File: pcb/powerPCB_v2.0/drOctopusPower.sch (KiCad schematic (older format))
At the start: 74 parts, among them CON1 Servo, CON10 AVR_Prog, CON2 Servo, CON3 Heater, CON4 +12V, CON5 BEC, CON6 PIN-2x2_angled, CON7 FAN1, CON8 FAN2, CON9 UART, Q1 16MHz, SW1 RESET, T1 IRLR2905PBF, T2 IRLML6244TRPBF, T3 IRLML6244TRPBF, T4 IRLML6244TRPBF, U1 ATmega328-AU, U2 78M05CDT, U3 ESP-01, U4 AMS1117-3.3

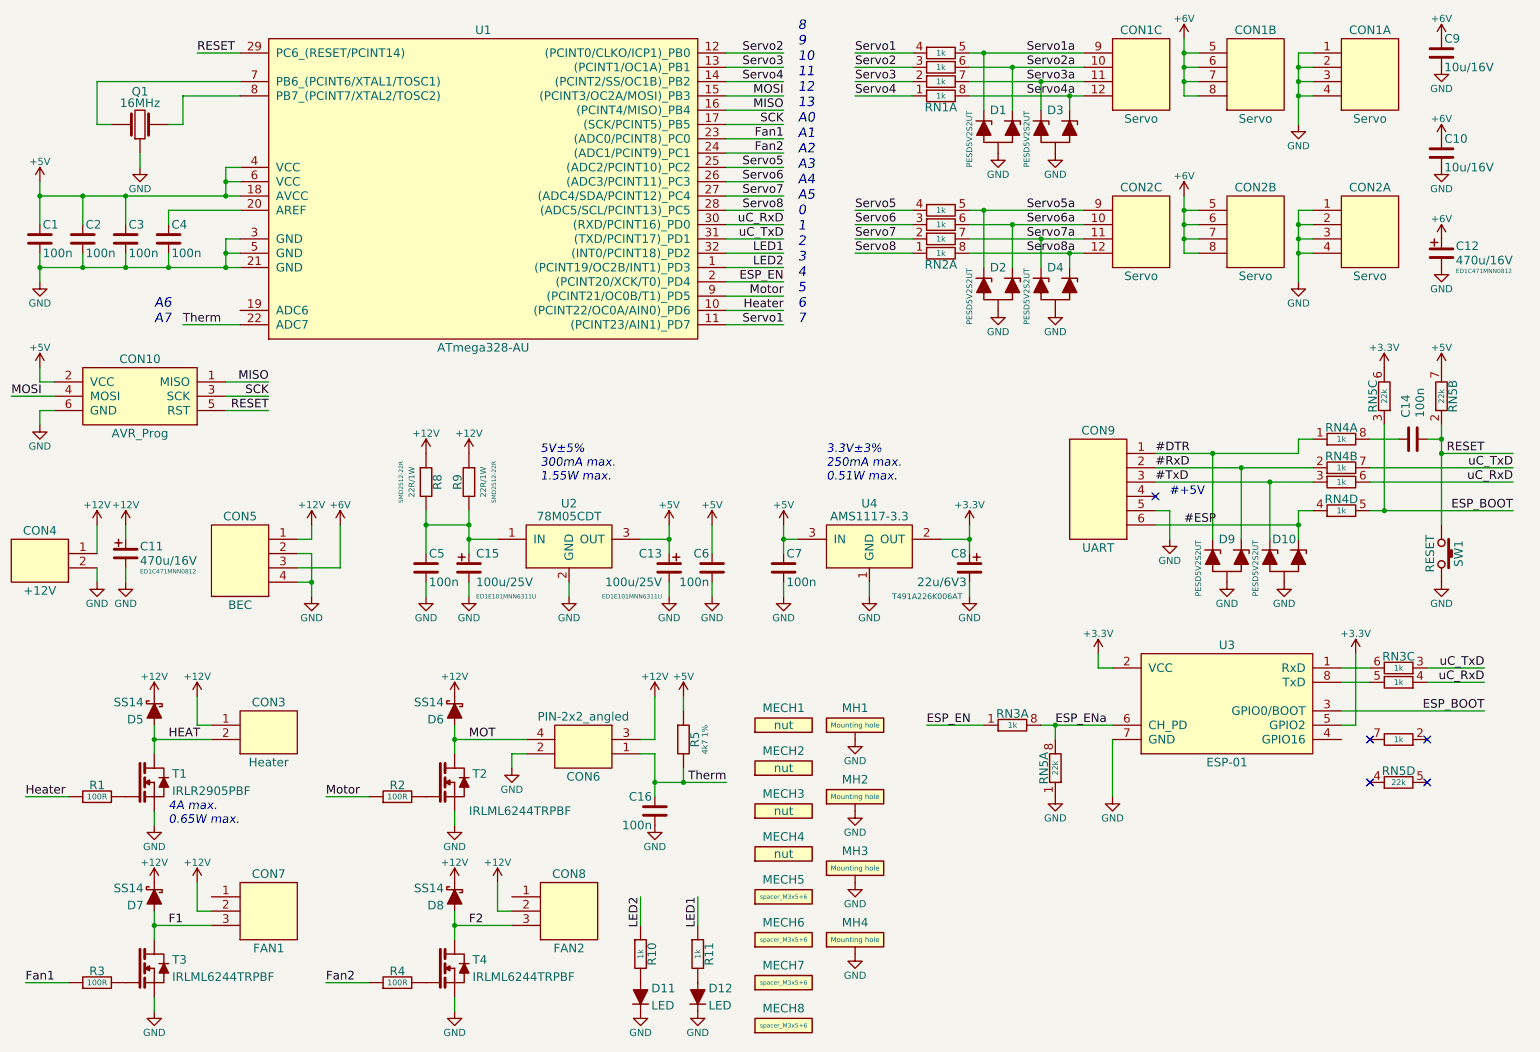
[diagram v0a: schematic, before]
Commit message: Working on Power PCB
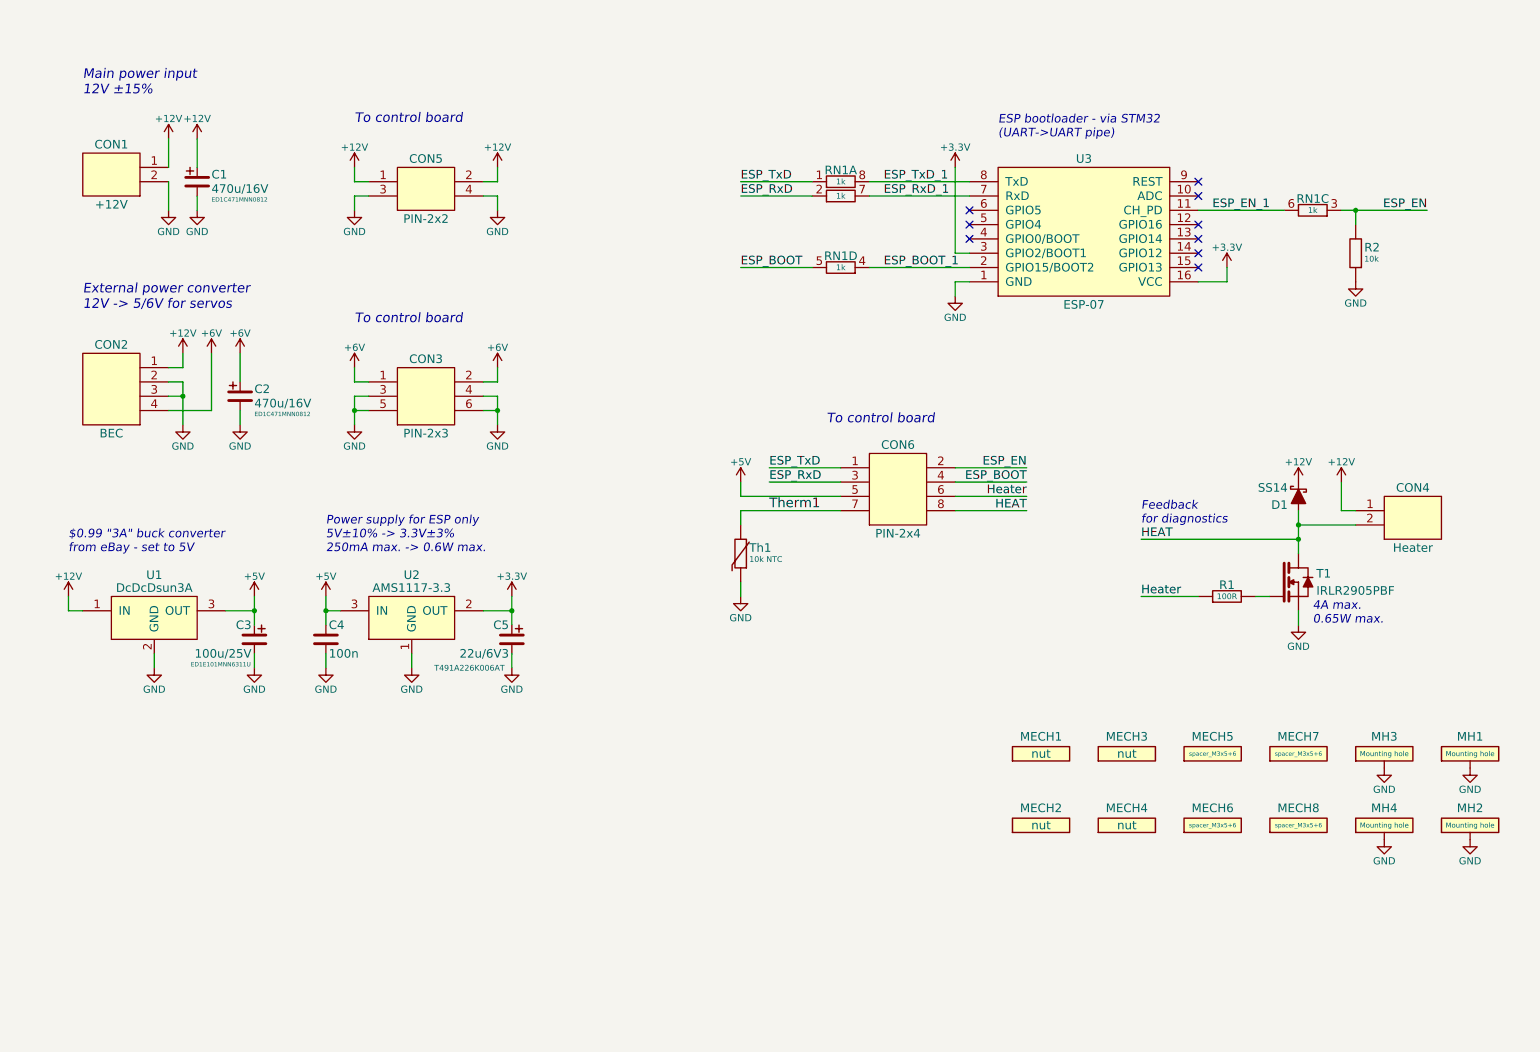
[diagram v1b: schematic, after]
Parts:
- removed C1, C14, C16, C2, C3, C4, C5, C6: 100n, 0603_N, symbol C
- removed C10, C9: 10u/16V, 0805_N, symbol C
- removed C12: 470u/16V, Cpol_8.0_12.0_M, symbol Cpol
- removed C13, C15: 100u/25V, Cpol_6.3_11.0_N, symbol Cpol
- removed CON1, CON2: Servo, PIN-3x4_angled_N, symbol PIN-3x4
- removed CON10: AVR_Prog, PIN-2x3_N, symbol AVR_Prog
- removed CON6: PIN-2x2_angled, PIN-2x2_angled_N, symbol PIN-2x2_angled
- removed CON7: FAN1, PIN-1x3_M, symbol PIN-1x3
- removed CON8: FAN2, PIN-1x3_M, symbol PIN-1x3
- removed CON9: UART, PIN-1x6_angled_N, symbol PIN-1x6_angled
- removed D1, D10, D2, D3, D4, D9: PESD5V2S2UT, SOT23-3_N, symbol PESD5V2S2UT
- removed D11, D12: LED, 0805_N, symbol diode
- removed D6, D7, D8: SS14, SMA_N, symbol SS14
- removed Q1: 16MHz, 3.7x3.1_N, symbol Ceramic_3.7x3.1_16MHz
- removed R10, R11: 1k, 0603_N, symbol R
- removed R2, R3, R4: 100R, 0603_N, symbol R
- removed R5: 4k7 1%, 0603_N, symbol R
- removed R8, R9: 22R/1W, 2512_N, symbol R
- removed RN1, RN2, RN4: 1k, 4x0603_N, symbol R_Network_4
- removed RN5: 22k, 4x0603_N, symbol R_Network_4
- removed SW1: RESET, MicroswitchSmd-4.3_N, symbol MicroswitchSmt-4.3
- removed T2, T3, T4: IRLML6244TRPBF, SOT23-3_N, symbol IRLML6244TRPBF
- removed U1: ATmega328-AU, QFP-32-0.8_M, symbol ATmega328-AU
- removed U2: 78M05CDT, D-PAK_N, symbol 78M05CDT
- removed U3: ESP-01, ESP-01_N_socket, symbol ESP-01
- added C2: 470u/16V, niceRLC:Cpol_8.0_12.0_HR_N, symbol Cpol
- added C3: 100u/25V, niceRLC:Cpol_6.3_11.0_HR_N, symbol Cpol
- added CON3: PIN-2x3, PIN-2x3_N, symbol PIN-2x3
- added CON5: PIN-2x2, PIN-2x2_N, symbol PIN-2x2
- added CON6: PIN-2x4, nicePinheaders:PIN-2x4_N, symbol PIN-2x4
- added R2: 10k, 0603_N, symbol R_V
- added Th1: 10k NTC, 0603_N, symbol Thermistor_V
- added U1: DcDcDsun3A, niceModules:DcDcDsun3A_5.08N, symbol DcDcDsun3A
- added U3: ESP-07, ESP-07_N, symbol ESP-07
- C1: renamed from C11; footprint Cpol_8.0_12.0_M -> niceRLC:Cpol_8.0_12.0_HR_N
- renumbered C7 to C4, C8 to C5, CON4 to CON1, CON5 to CON2, CON3 to CON4, D5 to D1, RN3 to RN1, U4 to U2
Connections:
- net +12V: now also CON5.1, CON5.2, U1.1 (IN)
- net +3V3: now also U3.16 (VCC), U3.3 (GPIO2/BOOT1)
- net +5V: now also C3.1, CON6.5, U1.3 (OUT)
- net +6V: now also CON2.4, C2.1, CON3.1, CON3.2; no longer CON2.3
- net ESP_BOOT: now also RN1.5 (2), CON6.4
- net ESP_EN: now also RN1.3 (1), CON6.2, R2.2; no longer RN1.1
- net GND: now also CON2.3, C2.2, C3.2, CON3.3, CON3.4, CON3.5, CON3.6, CON5.3, CON5.4, R2.1, Th1.1, U1.2 (GND), U3.1 (GND); no longer CON2.4
- net HEAT: now also CON6.8
- net Heater: now also CON6.6
- removed net ESP_ENa: RN1.8 (2)
- removed net uC_RxD: RN1.4 (1)
- removed net uC_TxD: RN1.3 (1)
- new net ESP_BOOT_1: RN1.4 (1), U3.2 (GPIO15/BOOT2)
- new net ESP_EN_1: RN1.6 (2), U3.11 (CH_PD)
- new net ESP_RxD: CON6.3, RN1.2 (1)
- new net ESP_RxD_1: RN1.7 (2), U3.7 (RxD)
- new net ESP_TxD: CON6.1, RN1.1
- new net ESP_TxD_1: RN1.8 (2), U3.8 (TxD)
- new net Therm1: CON6.7, Th1.2
- no-connect marks 5 -> 9
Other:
- note added: "$0.99 "3A" buck converter\nfrom eBay - set to 5V"
- note added: "ESP bootloader - via STM32 \n(UART->UART pipe)"
- note added: "External power converter\n12V -> 5/6V for servos"
- note added: "Feedback\nfor diagnostics"
- note added: "Main power input\n12V ±15%"
- note added: "Power supply for ESP only\n5V±10% -> 3.3V±3%\n250mA max. -> 0.6W max."
- note added: "To control board"
- note removed: "#+5V"
- note removed: "3.3V±3%\n250mA max.\n0.51W max."
- note removed: "5V±5%\n300mA max.\n1.55W max."
- note removed: "8\n9\n10\n11\n12\n13\nA0\nA1\nA2\nA3\nA4\nA5\n0\n1\n2\n3\n4\n5\n6\n7"
- note removed: "A6\nA7"
- moved on the sheet: C1, C4, C5, CON1, CON2, CON4, D1, MECH1, MECH2, MECH3, MECH4, MECH5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
